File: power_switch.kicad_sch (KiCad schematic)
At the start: 14 parts, among them Q1 NMOS, Q2 NMOS, Q3 NMOS

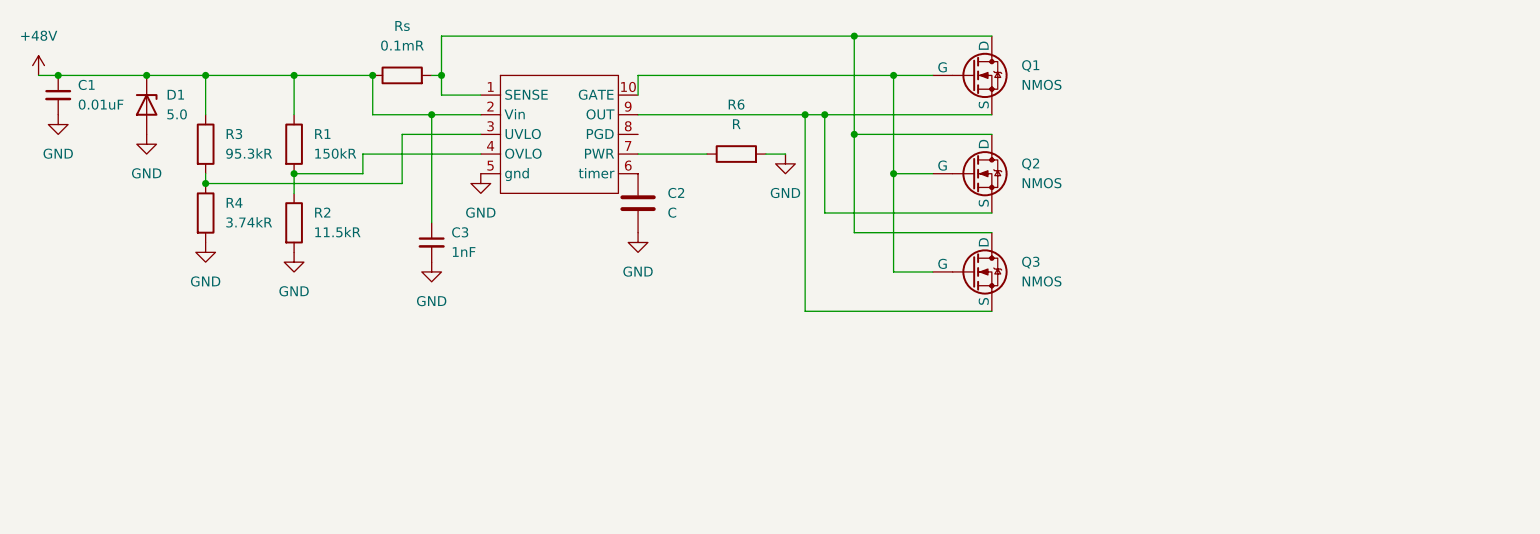
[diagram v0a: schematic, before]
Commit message: feat: added power switch schematics
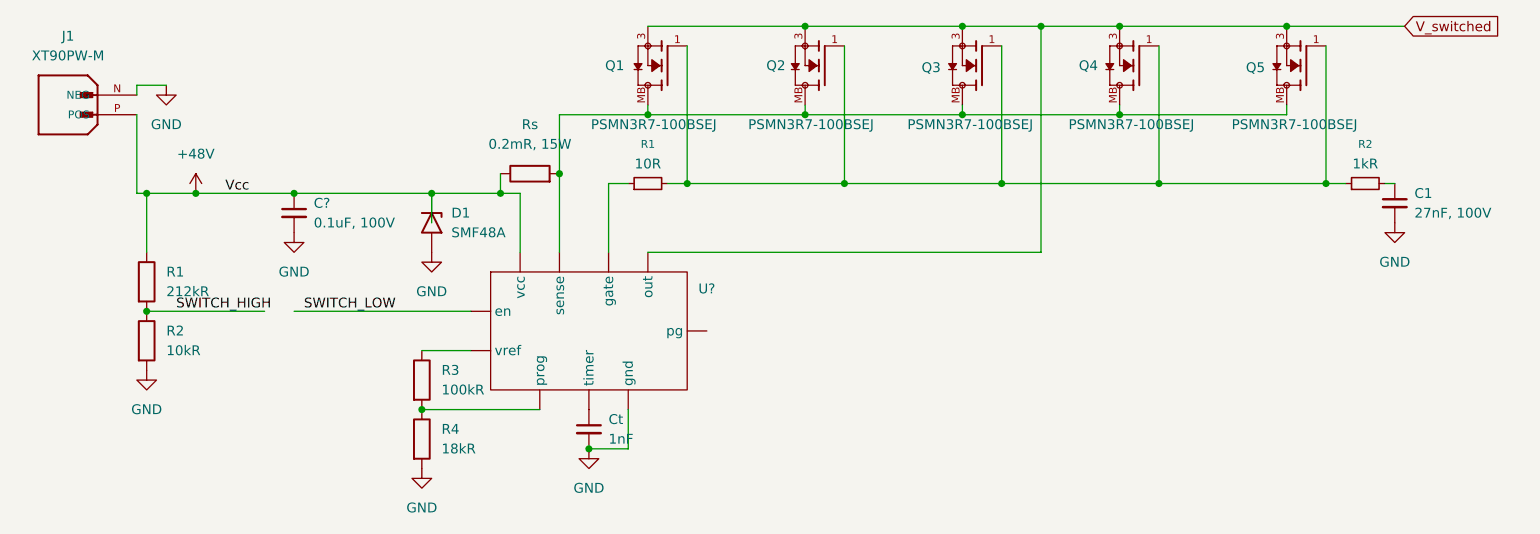
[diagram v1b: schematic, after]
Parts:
- removed C2: C, symbol Device:C
- removed C3: 1nF, symbol Device:C_Small
- removed D1: 5.0, symbol Device:D_Zener
- removed Q1, Q2, Q3: NMOS, symbol Simulation_SPICE:NMOS
- removed R6: R, symbol Device:R
- removed U1: ~, symbol symbols:LM5069
- added C?: 0.1uF, 100V, symbol Device:C_Small
- added Ct: 1nF, symbol Device:C_Small
- added D1: SMF48A, Package_SON:WSON-6-1EP_2x2mm_P0.65mm_EP1x1.6mm_ThermalVias, symbol Diode:SMF48A
- added J1: XT90PW-M, XT90PW-M:AMASS_XT90PW-M, symbol xt90:XT90PW-M
- added Q1, Q2, Q3, Q4, Q5: PSMN3R7-100BSEJ, PSMN3R7-100BSEJ:TRANS_PSMN3R7-100BSEJ, symbol PSMN3R7-100BSEJ:PSMN3R7-100BSEJ
- added R1: 10R, symbol Device:R_Small
- added R2: 1kR, symbol Device:R_Small
- added U?: ~, symbol symbols:_TPS2490
- C1: value 0.01uF -> 27nF, 100V
- R1: value 150kR -> 212kR
- R2: value 11.5kR -> 10kR
- R3: value 95.3kR -> 100kR
- R4: value 3.74kR -> 18kR
- Rs: value 0.1mR -> 0.2mR, 15W
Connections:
- net +48V: now also C?.1, D1.1 (A1), J1.P (POS), U?. (pg); no longer C1.1, R3.1
- net GND: now also C?.2, Ct.2, D1.2 (A2), J1.N (NEG), U?. (pg)
- net at Rs.2: now also Q1.MB, Q2.MB, Q3.MB, Q4.MB, Q5.MB, U?. (pg)
- net SWITCH_HIGH: now reaches R1.2, R2.1
- net at R3.2, R4.1: now also U?. (pg)
- new net: Q1.1, Q2.1, Q3.1, Q4.1, Q5.1, R1.2, R2.1
- new net: C1.1, R2.2
- new net: R1.1, U?. (pg)
- new net: Ct.1, U?. (pg)
- new net: R3.1, U?. (pg)
- new net SWITCH_LOW: U?. (pg)
- new net V_switched: Q1.3, Q2.3, Q3.3, Q4.3, Q5.3, U?. (pg)
